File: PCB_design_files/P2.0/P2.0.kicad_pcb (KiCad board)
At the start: 4 copper layers, 20 x 20 mm, 0 parts

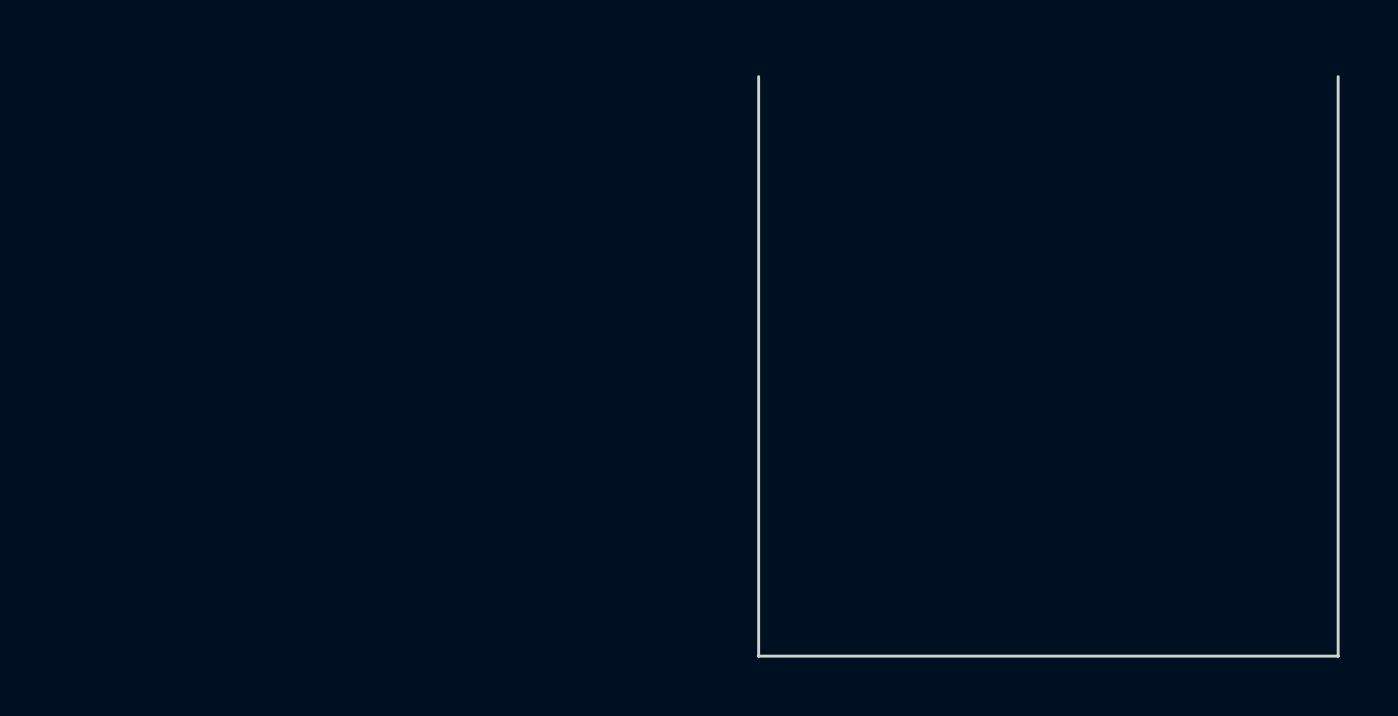
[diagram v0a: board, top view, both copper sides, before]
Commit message: Updated P2.0
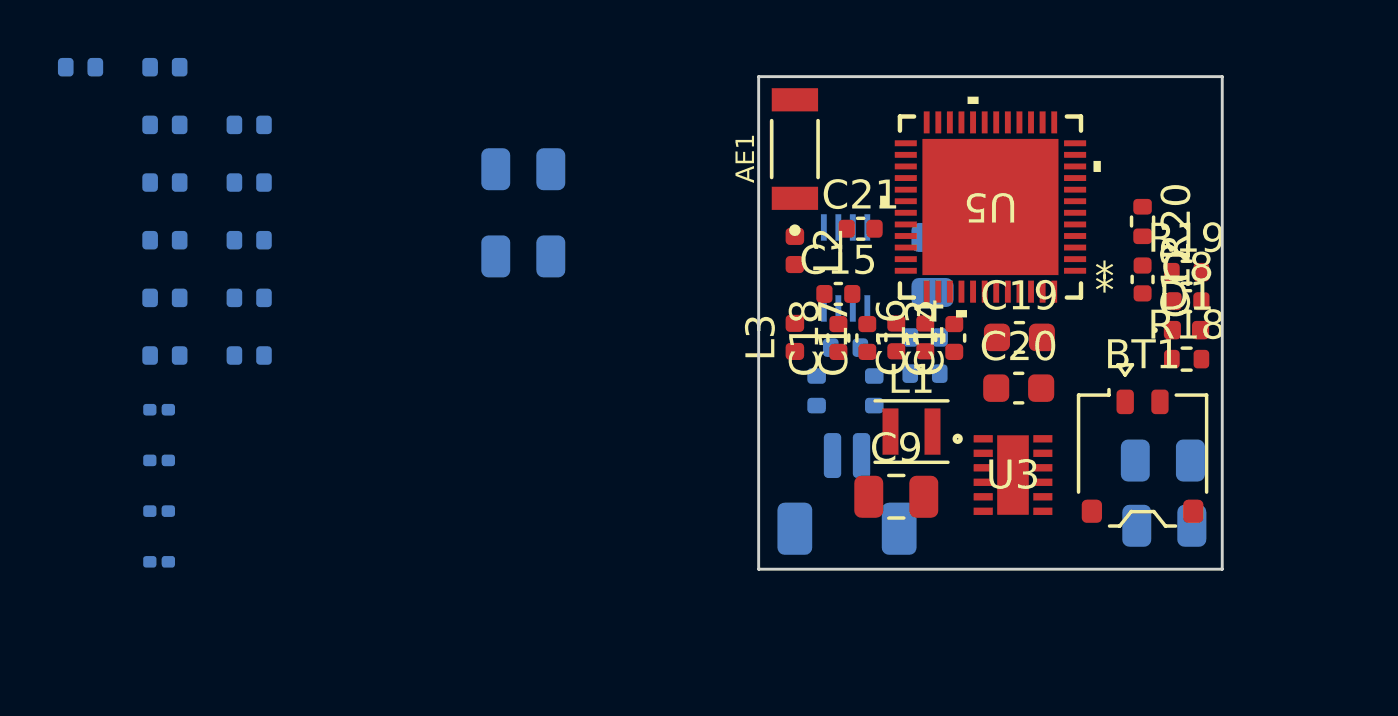
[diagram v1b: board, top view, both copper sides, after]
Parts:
- added AE1: Antenna_Chip, Library:XDCR_2450AT18B100E, F.Cu at (76.2, 34.5)
- added BT1: BHSD-1225-SM, Connector_JST:JST_ACH_BM02B-ACHSS-GAN-ETF_1x02-1MP_P1.20mm_Vertical, F.Cu at (88.2, 45.1)
- added C1: 10uF, Capacitor_SMD:C_0805_2012Metric, B.Cu at (81.0, 38.5)
- added C10: 1uF, Capacitor_SMD:C_0805_2012Metric, B.Cu at (89.0, 47.5)
- added C11: 1uF, Capacitor_SMD:C_0805_2012Metric, B.Cu at (89.0, 45.2)
- added C12: 100nF, Capacitor_SMD:C_0402_1005Metric, F.Cu at (88.2, 39.0)
- added C13: 100nF, Capacitor_SMD:C_0402_1005Metric, F.Cu at (81.8, 41.0)
- added C14: 100nF, Capacitor_SMD:C_0402_1005Metric, F.Cu at (79.8, 41.0)
- added C15: 1.2pF, Capacitor_SMD:C_0402_1005Metric, F.Cu at (77.8, 39.5)
- added C16: 12pF, Capacitor_SMD:C_0402_1005Metric, F.Cu at (80.8, 41.0)
- added C17: 100pF, Capacitor_SMD:C_0402_1005Metric, F.Cu at (78.8, 41.0)
- added C18: 12pF, Capacitor_SMD:C_0402_1005Metric, F.Cu at (77.8, 41.0)
- added C19: 1uF, Capacitor_SMD:C_0603_1608Metric, F.Cu at (84.0, 41.0)
- added C2: 10uF, Capacitor_SMD:C_0805_2012Metric, B.Cu at (66.9, 35.2)
- added C20: 4.7uF, Capacitor_SMD:C_0603_1608Metric, F.Cu at (84.0, 42.8)
- added C21: N.C., Capacitor_SMD:C_0402_1005Metric, F.Cu at (78.5, 37.2)
- added C3: 0.1uF, Capacitor_SMD:C_0201_0603Metric, B.Cu at (54.3, 43.5)
- added C4: 0.1uF, Capacitor_SMD:C_0201_0603Metric, B.Cu at (54.3, 45.2)
- added C5: 0.1uF, Capacitor_SMD:C_0201_0603Metric, B.Cu at (54.3, 47.0)
- added C6: 10nF, Capacitor_SMD:C_0201_0603Metric, B.Cu at (54.3, 48.7)
- added C7: 10uF, Capacitor_SMD:C_0805_2012Metric, B.Cu at (66.9, 38.2)
- added C8: 2.2uF, Capacitor_SMD:C_0402_1005Metric, F.Cu at (89.8, 39.8)
- added C9: 33uF, Capacitor_SMD:C_0805_2012Metric, F.Cu at (79.8, 46.5)
- added D1: LED, LED_SMD:LED_0402_1005Metric, F.Cu at (89.8, 40.8)
- added J1: EEG_IN, Connector_JST:JST_SH_BM02B-SRSS-TB_1x02-1MP_P1.00mm_Vertical, B.Cu at (78.0, 46.4)
- added L1: 2.2uH, Inductor_SMD:L_Murata_DFE201610P, F.Cu at (80.3, 44.2)
- added L2: 3.3nH, Inductor_SMD:L_0402_1005Metric, F.Cu at (76.2, 38.0)
- added L3: 2.7nH, Inductor_SMD:L_0402_1005Metric, F.Cu at (76.2, 41.0)
- added R1: 68k, Resistor_SMD:R_0402_1005Metric, B.Cu at (79.0, 42.8)
- added R10: 604, Resistor_SMD:R_0402_1005Metric, B.Cu at (57.4, 41.6)
- added R11: 16k, Resistor_SMD:R_0402_1005Metric, B.Cu at (54.5, 31.7)
- added R12: 2.49k, Resistor_SMD:R_0402_1005Metric, B.Cu at (54.5, 33.7)
- added R13: 49.9k, Resistor_SMD:R_0402_1005Metric, B.Cu at (54.5, 35.7)
- added R14: 10k, Resistor_SMD:R_0402_1005Metric, B.Cu at (54.5, 37.6)
- added R15: 100k, Resistor_SMD:R_0402_1005Metric, B.Cu at (54.5, 39.6)
- added R16: 100k, Resistor_SMD:R_0402_1005Metric, B.Cu at (54.5, 41.6)
- added R17: ?150k, Resistor_SMD:R_0402_1005Metric, B.Cu at (51.6, 31.7)
- added R18: 1.1k, Resistor_SMD:R_0402_1005Metric, F.Cu at (89.8, 41.8)
- added R19: 1.1k, Resistor_SMD:R_0402_1005Metric, F.Cu at (89.8, 38.8)
- added R2: 68k, Resistor_SMD:R_0402_1005Metric, B.Cu at (77.0, 42.8)
- added R20: 10k, Resistor_SMD:R_0402_1005Metric, F.Cu at (88.2, 37.0)
- added R3: 8.2k, Resistor_SMD:R_0402_1005Metric, B.Cu at (78.0, 41.4)
- added R4: 100k, Resistor_SMD:R_0402_1005Metric, B.Cu at (80.8, 41.0)
- added R5: 1k, Resistor_SMD:R_0402_1005Metric, B.Cu at (80.7, 42.2)
- added R6: ?100k, Resistor_SMD:R_0402_1005Metric, B.Cu at (57.4, 33.7)
- added R7: 1k, Resistor_SMD:R_0402_1005Metric, B.Cu at (57.4, 35.7)
- added R8: 100k, Resistor_SMD:R_0402_1005Metric, B.Cu at (57.4, 37.6)
- added R9: 100k, Resistor_SMD:R_0402_1005Metric, B.Cu at (57.4, 39.6)
- added U1: INA819IDRGR, Library:SON_9IDRGR_TEX, B.Cu at (78.0, 38.6)
- added U3: TPS61094, Library:TPS61094DSSR, F.Cu at (83.8, 45.7)
- added U5: NRF52832-QFAA-R, Library:QFN-48_NOR, F.Cu at (83.0, 36.5)
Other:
- board size 20 x 20 mm -> 16 x 17 mm

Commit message: Updated schematic
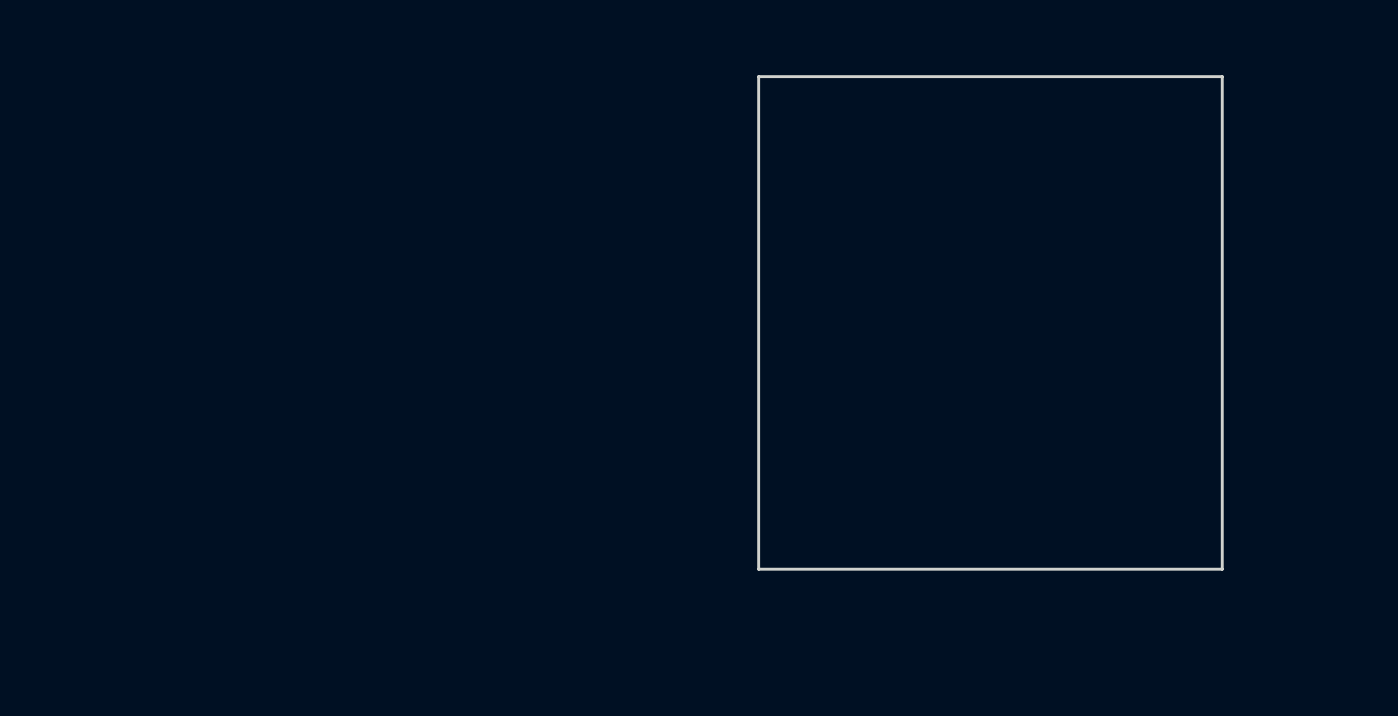
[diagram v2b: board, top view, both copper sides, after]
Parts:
- removed AE1: Antenna_Chip, Library:XDCR_2450AT18B100E
- removed BT1: BHSD-1225-SM, Connector_JST:JST_ACH_BM02B-ACHSS-GAN-ETF_1x02-1MP_P1.20mm_Vertical
- removed C1, C2, C7: 10uF, Capacitor_SMD:C_0805_2012Metric
- removed C10, C11: 1uF, Capacitor_SMD:C_0805_2012Metric
- removed C12, C13, C14: 100nF, Capacitor_SMD:C_0402_1005Metric
- removed C15: 1.2pF, Capacitor_SMD:C_0402_1005Metric
- removed C16, C18: 12pF, Capacitor_SMD:C_0402_1005Metric
- removed C17: 100pF, Capacitor_SMD:C_0402_1005Metric
- removed C19: 1uF, Capacitor_SMD:C_0603_1608Metric
- removed C20: 4.7uF, Capacitor_SMD:C_0603_1608Metric
- removed C21: N.C., Capacitor_SMD:C_0402_1005Metric
- removed C3, C4, C5: 0.1uF, Capacitor_SMD:C_0201_0603Metric
- removed C6: 10nF, Capacitor_SMD:C_0201_0603Metric
- removed C8: 2.2uF, Capacitor_SMD:C_0402_1005Metric
- removed C9: 33uF, Capacitor_SMD:C_0805_2012Metric
- removed D1: LED, LED_SMD:LED_0402_1005Metric
- removed J1: EEG_IN, Connector_JST:JST_SH_BM02B-SRSS-TB_1x02-1MP_P1.00mm_Vertical
- removed L1: 2.2uH, Inductor_SMD:L_Murata_DFE201610P
- removed L2: 3.3nH, Inductor_SMD:L_0402_1005Metric
- removed L3: 2.7nH, Inductor_SMD:L_0402_1005Metric
- removed R1, R2: 68k, Resistor_SMD:R_0402_1005Metric
- removed R10: 604, Resistor_SMD:R_0402_1005Metric
- removed R11: 16k, Resistor_SMD:R_0402_1005Metric
- removed R12: 2.49k, Resistor_SMD:R_0402_1005Metric
- removed R13: 49.9k, Resistor_SMD:R_0402_1005Metric
- removed R14, R20: 10k, Resistor_SMD:R_0402_1005Metric
- removed R15, R16, R4, R8, R9: 100k, Resistor_SMD:R_0402_1005Metric
- removed R17: ?150k, Resistor_SMD:R_0402_1005Metric
- removed R18, R19: 1.1k, Resistor_SMD:R_0402_1005Metric
- removed R3: 8.2k, Resistor_SMD:R_0402_1005Metric
- removed R5, R7: 1k, Resistor_SMD:R_0402_1005Metric
- removed R6: ?100k, Resistor_SMD:R_0402_1005Metric
- removed U1: INA819IDRGR, Library:SON_9IDRGR_TEX
- removed U3: TPS61094, Library:TPS61094DSSR
- removed U5: NRF52832-QFAA-R, Library:QFN-48_NOR
